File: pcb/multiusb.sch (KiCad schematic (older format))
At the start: 11 parts, among them P1 USB_MICRO_OTG, P2 USB_MINI_OTG, P3 USB_A

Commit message: updated USB A footprint
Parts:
- P1: footprint Connectors:USB_Micro-B -> Connectors:USB_Micro-B_10103594-0001LF
- P3: footprint Connectors:USB_A -> project:USB_A
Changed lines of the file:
@@
 LIBS:contrib
 LIBS:valves
+LIBS:multiusb-cache
 EELAYER 25 0
 EELAYER END
@@
 F 0 "P1" H 2975 2825 50  0000 C CNN
 F 1 "USB_MICRO_OTG" H 2650 3150 50  0000 C CNN
-F 2 "Connectors:USB_Micro-B" V 2600 2850 50  0001 C CNN
+F 2 "Connectors:USB_Micro-B_10103594-0001LF" V 2600 2850 50  0001 C CNN
 F 3 "" V 2600 2850 50  0000 C CNN
 	1    2650 2950
@@
 F 0 "P3" H 5050 2750 50  0000 C CNN
 F 1 "USB_A" H 4800 3150 50  0000 C CNN
-F 2 "Connectors:USB_A" V 4800 2850 50  0001 C CNN
+F 2 "project:USB_A" V 4800 2850 50  0001 C CNN
 F 3 "" V 4800 2850 50  0000 C CNN
 	1    4850 2950

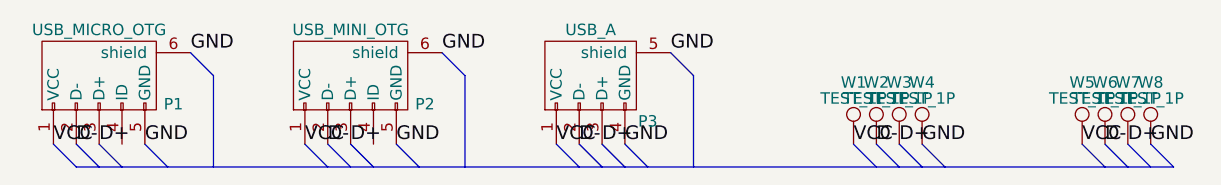
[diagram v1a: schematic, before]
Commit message: getting close to the final pcb layout
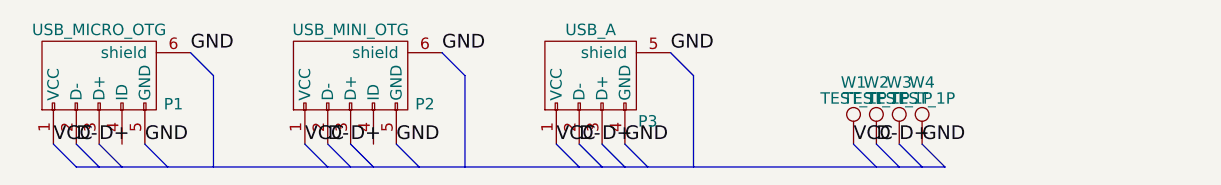
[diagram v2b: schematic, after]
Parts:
- removed W5, W6, W7, W8: TEST_1P, Mounting_Holes:MountingHole_3mm_Pad, symbol TEST_1P
- W1: footprint Mounting_Holes:MountingHole_3mm_Pad -> Mounting_Holes:MountingHole_2.5mm_Pad
- W2, W3, W4: footprint Mounting_Holes:MountingHole_3mm_Pad -> Mounting_Holes:MountingHole_2.5mm_Pad_Via
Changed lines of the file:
@@
 	3050 2850 3150 2950
-Wire Bus Line
-	2550 3350 7350 3350
 Wire Bus Line
 	3150 2950 3150 3350
@@
 Text Label 5950 3250 0    60   ~ 0
 VCC
-Entry Bus Bus
-	6950 3250 7050 3350
-Entry Bus Bus
-	7050 3250 7150 3350
-Entry Bus Bus
-	7150 3250 7250 3350
-Entry Bus Bus
-	7250 3250 7350 3350
-Text Label 7250 3250 0    60   ~ 0
-GND
-Text Label 7150 3250 0    60   ~ 0
-D+
-Text Label 7050 3250 0    60   ~ 0
-D-
-Text Label 6950 3250 0    60   ~ 0
-VCC
 $Comp
 L TEST_1P W1
@@
 F 0 "W1" H 5950 3520 50  0000 C CNN
 F 1 "TEST_1P" H 5950 3450 50  0000 C CNN
-F 2 "Mounting_Holes:MountingHole_3mm_Pad" H 6150 3250 50  0001 C CNN
+F 2 "Mounting_Holes:MountingHole_2.5mm_Pad" H 6150 3250 50  0001 C CNN
 F 3 "" H 6150 3250 50  0000 C CNN
 	1    5950 3250
@@
 F 0 "W2" H 6050 3520 50  0000 C CNN
 F 1 "TEST_1P" H 6050 3450 50  0000 C CNN
-F 2 "Mounting_Holes:MountingHole_3mm_Pad" H 6250 3250 50  0001 C CNN
+F 2 "Mounting_Holes:MountingHole_2.5mm_Pad_Via" H 6250 3250 50  0001 C CNN
 F 3 "" H 6250 3250 50  0000 C CNN
 	1    6050 3250
@@
 F 0 "W3" H 6150 3520 50  0000 C CNN
 F 1 "TEST_1P" H 6150 3450 50  0000 C CNN
-F 2 "Mounting_Holes:MountingHole_3mm_Pad" H 6350 3250 50  0001 C CNN
+F 2 "Mounting_Holes:MountingHole_2.5mm_Pad_Via" H 6350 3250 50  0001 C CNN
 F 3 "" H 6350 3250 50  0000 C CNN
 	1    6150 3250
@@
 F 0 "W4" H 6250 3520 50  0000 C CNN
 F 1 "TEST_1P" H 6250 3450 50  0000 C CNN
-F 2 "Mounting_Holes:MountingHole_3mm_Pad" H 6450 3250 50  0001 C CNN
+F 2 "Mounting_Holes:MountingHole_2.5mm_Pad_Via" H 6450 3250 50  0001 C CNN
 F 3 "" H 6450 3250 50  0000 C CNN
 	1    6250 3250
 	1    0    0    -1
 $EndComp
-$Comp
-L TEST_1P W5
-U 1 1 584DA4BF
-P 6950 3250
-F 0 "W5" H 6950 3520 50  0000 C CNN
-F 1 "TEST_1P" H 6950 3450 50  0000 C CNN
-F 2 "Mounting_Holes:MountingHole_3mm_Pad" H 7150 3250 50  0001 C CNN
-F 3 "" H 7150 3250 50  0000 C CNN
-	1    6950 3250
-	1    0    0    -1
-$EndComp
-$Comp
-L TEST_1P W6
-U 1 1 584DA505
-P 7050 3250
-F 0 "W6" H 7050 3520 50  0000 C CNN
-F 1 "TEST_1P" H 7050 3450 50  0000 C CNN
-F 2 "Mounting_Holes:MountingHole_3mm_Pad" H 7250 3250 50  0001 C CNN
-F 3 "" H 7250 3250 50  0000 C CNN
-	1    7050 3250
-	1    0    0    -1
-$EndComp
-$Comp
-L TEST_1P W7
-U 1 1 584DA530
-P 7150 3250
-F 0 "W7" H 7150 3520 50  0000 C CNN
-F 1 "TEST_1P" H 7150 3450 50  0000 C CNN
-F 2 "Mounting_Holes:MountingHole_3mm_Pad" H 7350 3250 50  0001 C CNN
-F 3 "" H 7350 3250 50  0000 C CNN
-	1    7150 3250
-	1    0    0    -1
-$EndComp
-$Comp
-L TEST_1P W8
-U 1 1 584DA55E
-P 7250 3250
-F 0 "W8" H 7250 3520 50  0000 C CNN
-F 1 "TEST_1P" H 7250 3450 50  0000 C CNN
-F 2 "Mounting_Holes:MountingHole_3mm_Pad" H 7450 3250 50  0001 C CNN
-F 3 "" H 7450 3250 50  0000 C CNN
-	1    7250 3250
-	1    0    0    -1
-$EndComp
+Wire Bus Line
+	2550 3350 6350 3350
 $EndSCHEMATC
